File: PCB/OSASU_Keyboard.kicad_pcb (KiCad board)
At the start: 2 copper layers, 62.3 x 19.2 mm, 23 parts, among them J1 Conn_01x05_Pin, J2 Conn_01x05_Socket, J3 Conn_01x05_Pin, J5 Conn_01x03, J6 Conn_01x05_Socket, P1 USB_C_Plug_USB2.0, SW2 SW_Push, U1 CH552T, U2 CH32V003FxPx

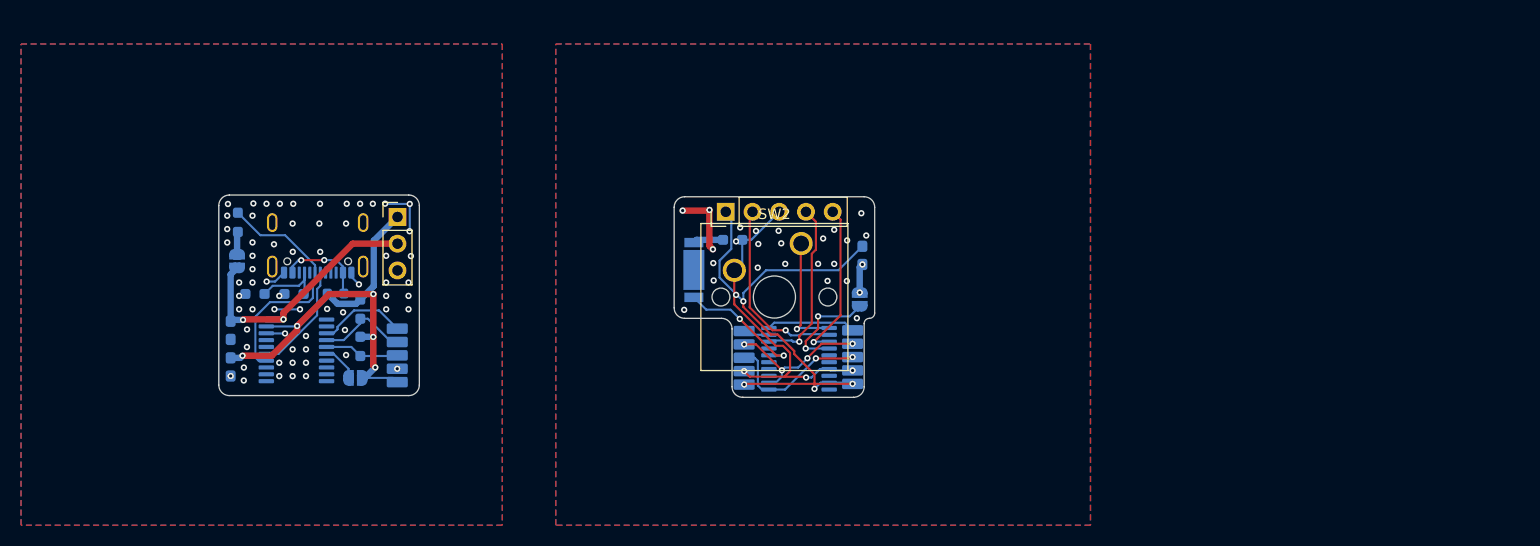
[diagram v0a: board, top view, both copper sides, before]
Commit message: commit
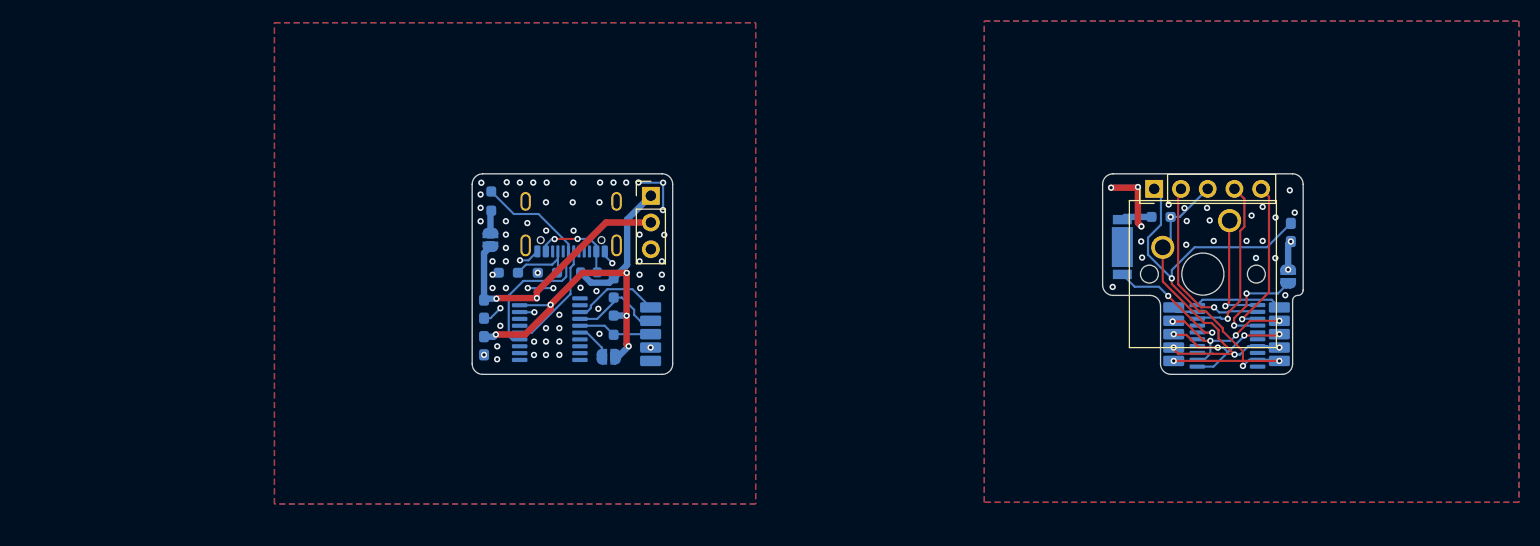
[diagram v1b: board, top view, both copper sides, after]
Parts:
- moved J2 40.9 mm to (220.8, 126.6)
- moved U2 40.8 mm to (226.4, 129.3)
- moved C3 40.8 mm to (232.4, 119.5)
- moved D1 40.8 mm to (216.4, 120.9)
- moved J6 40.8 mm to (219.4, 115.4)
- moved JP3 40.8 mm to (232.1, 123.7)
- moved R6 40.8 mm to (220.1, 118.0)
- moved SW2 40.8 mm to (226.6, 118.4)
- moved J3 40.6 mm to (231.8, 131.7)
- moved C1 24.2 mm to (155.7, 126.8)
- moved C2 24.2 mm to (155.7, 130.3)
- moved F1 24.2 mm to (165.7, 123.3)
- moved JP1 24.2 mm to (156.4, 120.2)
- moved JP2 24.2 mm to (167.6, 131.3)
- moved R3 24.2 mm to (156.4, 116.5)
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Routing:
- net /Sleve/Adress(Slave): track 2.50 -> 7.32 mm
- net +5V: track 45.8 -> 42.4 mm
- net GND: track 12.6 -> 14.2 mm
- net /Sleve/PC1: track 14.2 -> 15.1 mm, vias 2 -> 4
- net GND_{Slave}: track 40.9 -> 41.3 mm, vias 31 -> 30
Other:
- board size 62.3 x 19.2 mm -> 78.9 x 19 mm
- board text added: "3V3"
- board text added: "5V"
- board text added: "DFU"
- board text added: "FUSE"
- board text added: "GND"
- board text added: "RST"
- board text added: "RX"
- board text added: "SWDIO"
- board text added: "TX"
